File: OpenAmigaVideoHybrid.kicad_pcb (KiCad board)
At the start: 2 copper layers, 56.4 x 21.2 mm, 59 parts, among them J1 CONN_MAINBOARD, J2 SVIDEO_OUT, Q1 2N3904, Q2 2N3904, Q3 2N3904, Q4 2N3904, U1 AD724, Y1 4.433619M

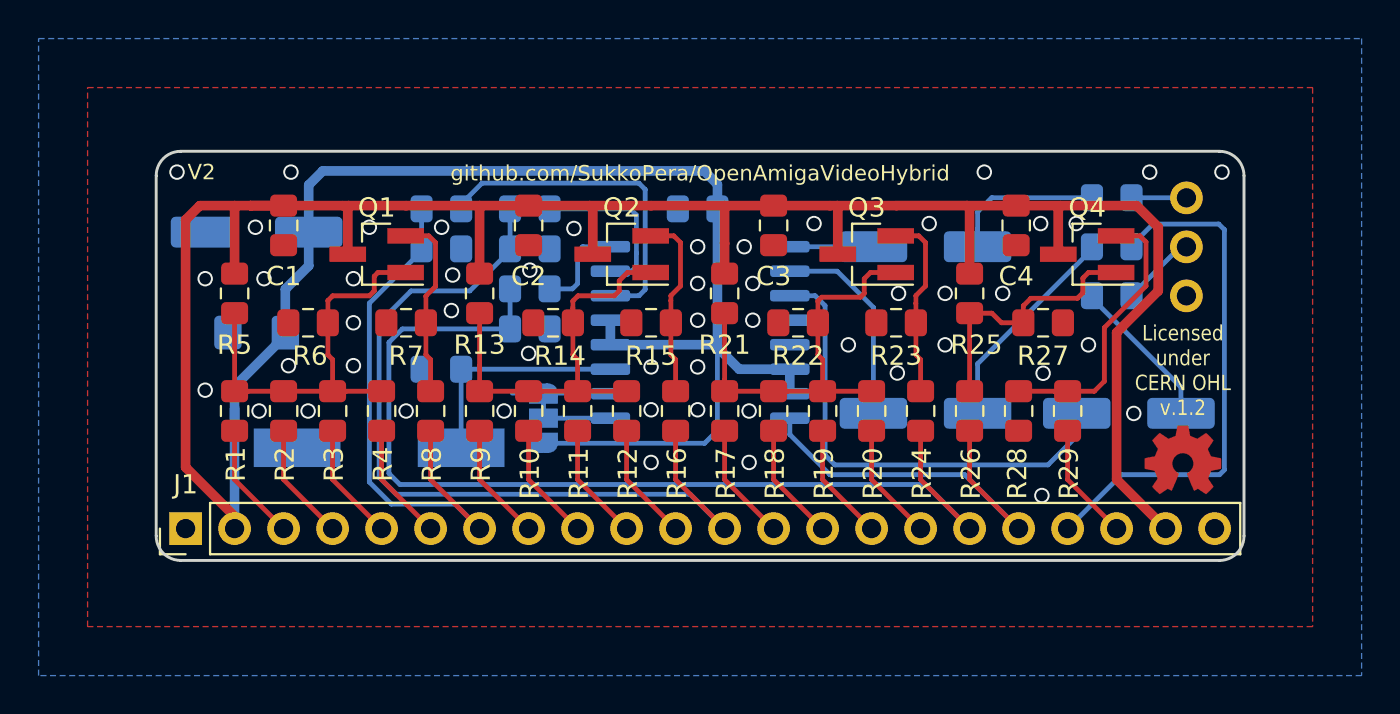
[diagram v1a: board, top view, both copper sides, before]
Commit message: I think we can call this good
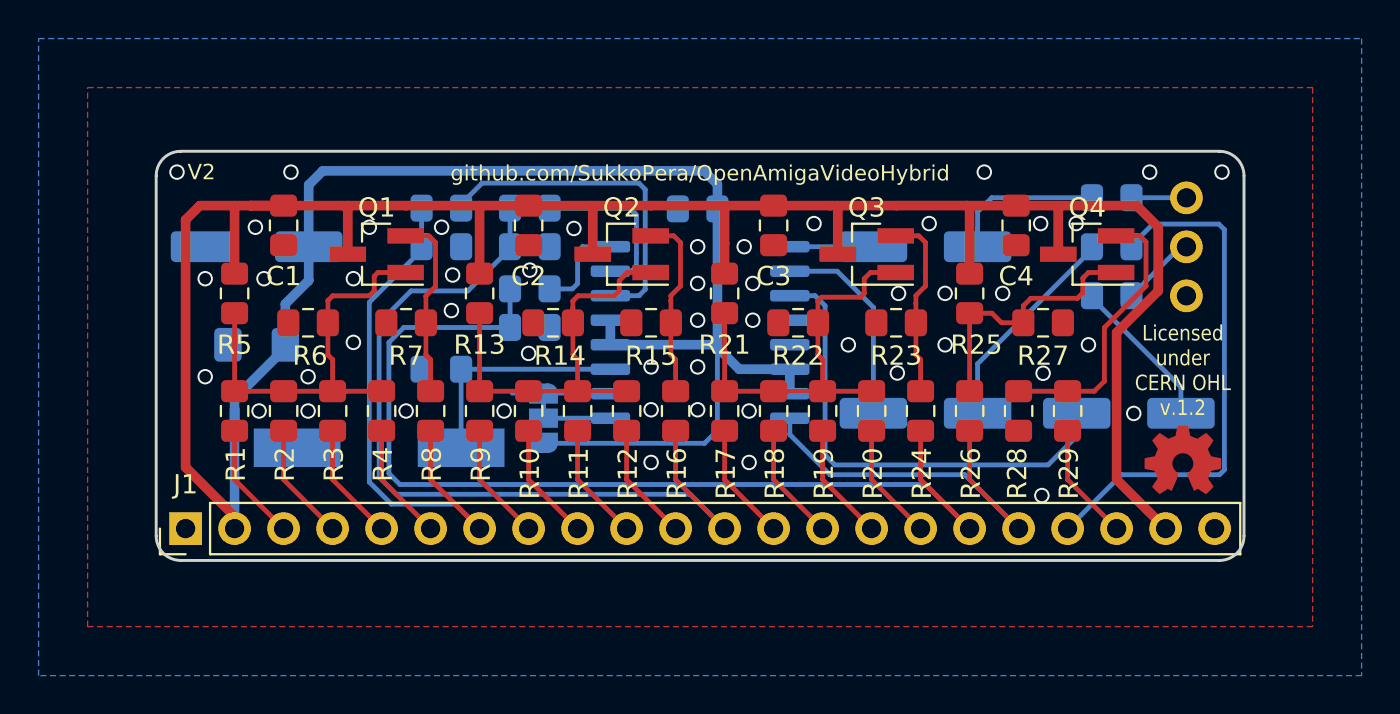
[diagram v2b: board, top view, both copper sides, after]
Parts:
- moved C13 0.76 mm to (123.1, 109.8)
- moved C14 0.64 mm to (123.1, 114.9)
- moved R30 0.11 mm to (132.6, 109.8)
- moved R31 0.11 mm to (137.2, 109.8)
- moved R32 0.07 mm to (137.2, 114.0)
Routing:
- net GND: vias 51 -> 50
